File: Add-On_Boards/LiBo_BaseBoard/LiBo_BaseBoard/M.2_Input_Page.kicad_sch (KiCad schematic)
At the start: 9 parts, among them J2 2199230-3

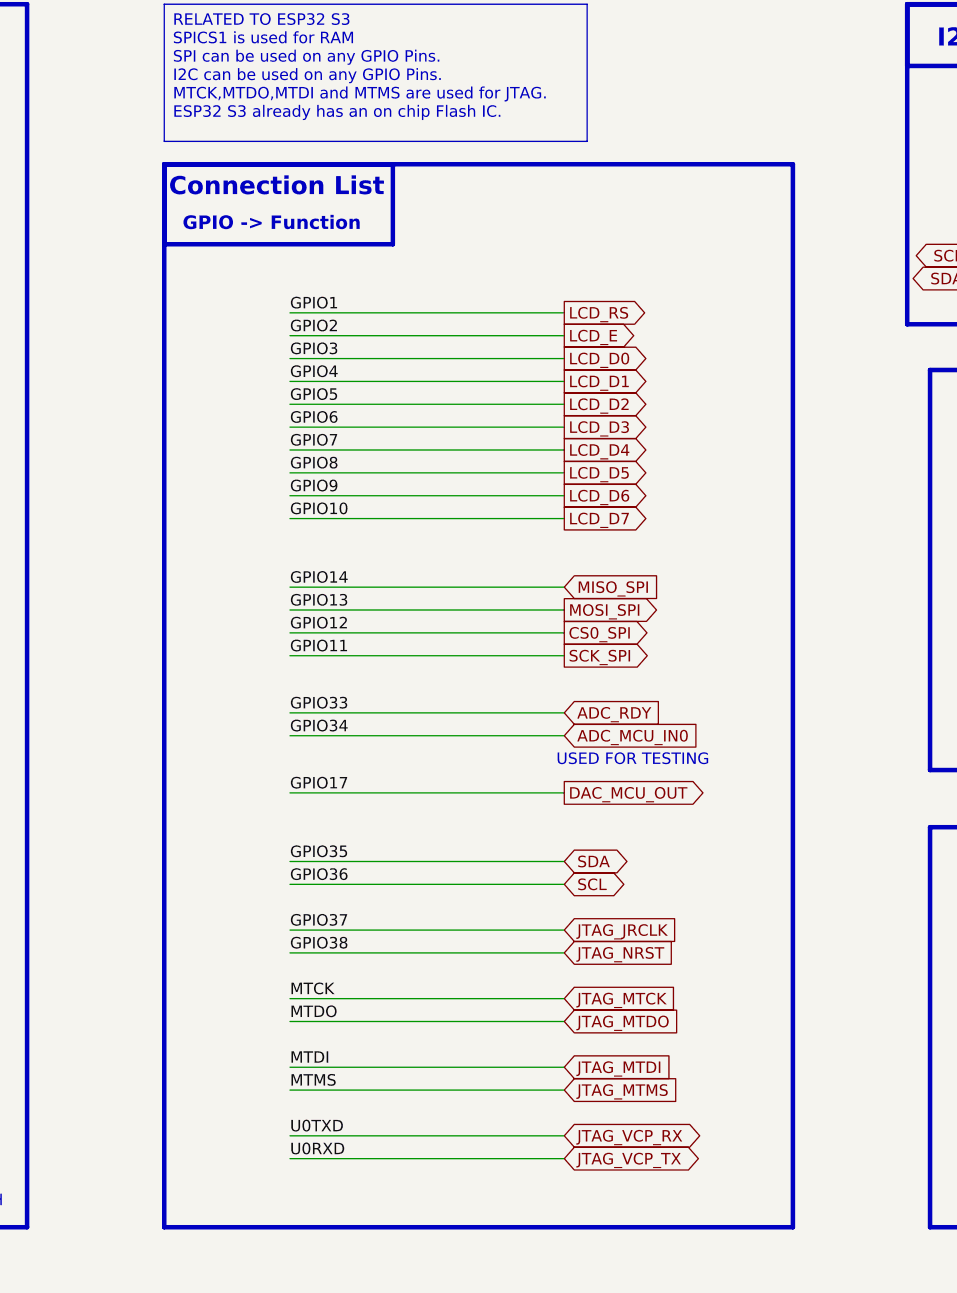
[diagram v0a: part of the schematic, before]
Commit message: first release
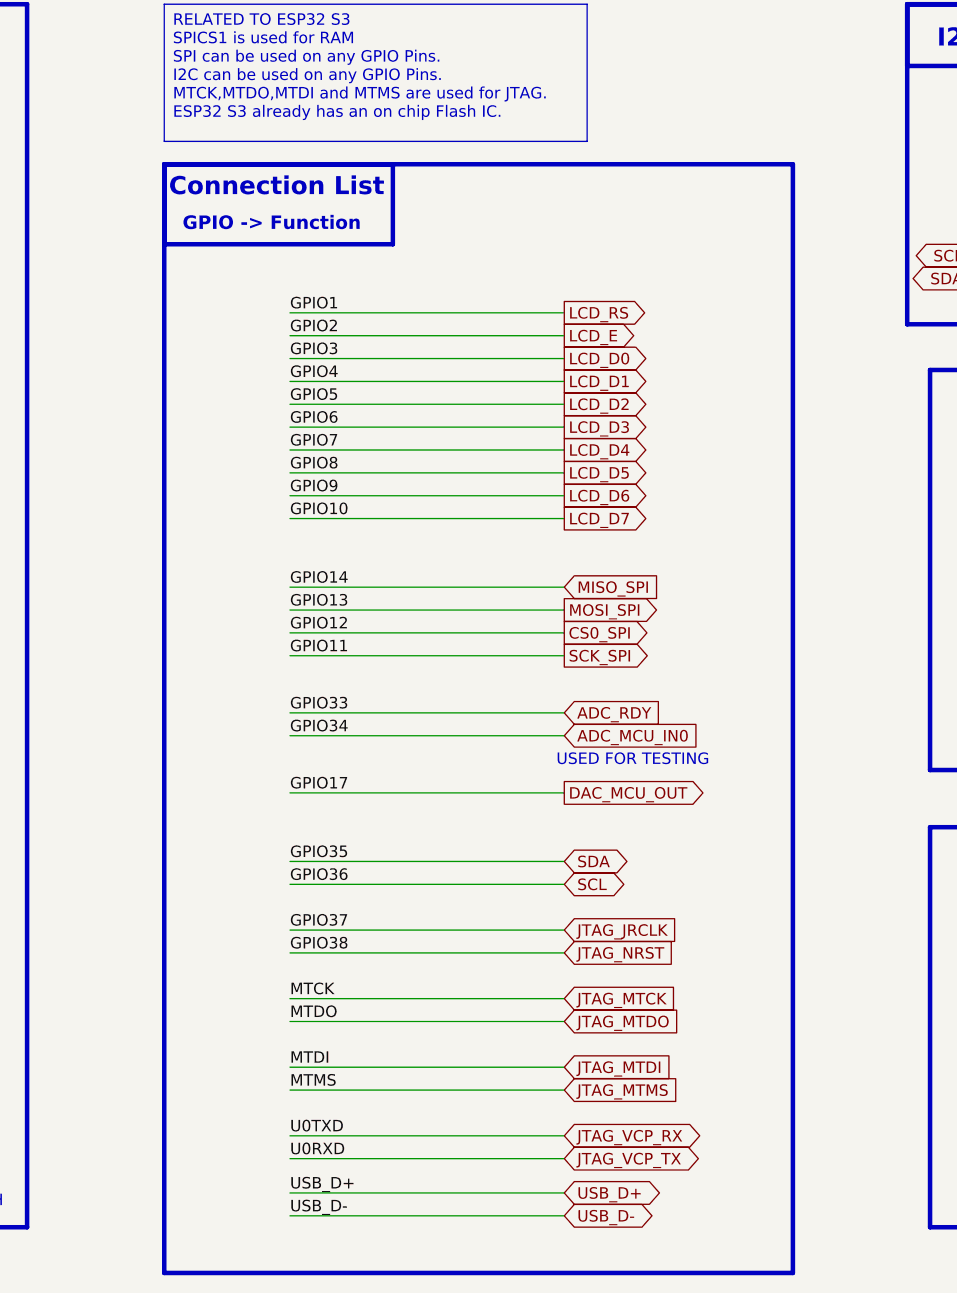
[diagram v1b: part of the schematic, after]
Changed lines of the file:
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@@
 	(rectangle
 		(start 128.27 39.37)
-		(end 198.12 157.48)
+		(end 198.12 162.56)
 		(stroke
 			(width 0.5)
@@
 	(wire
 		(pts
+			(xy 142.24 153.67) (xy 172.72 153.67)
+		)
+		(stroke
+			(width 0)
+			(type default)
+		)
+	)
+	(wire
+		(pts
 			(xy 81.28 80.01) (xy 81.28 72.39)
 		)
@@
 		(pts
 			(xy 53.34 52.07) (xy 53.34 54.61)
+		)
+		(stroke
+			(width 0)
+			(type default)
+		)
+	)
+	(wire
+		(pts
+			(xy 142.24 156.21) (xy 172.72 156.21)
 		)
 		(stroke
@@
 		)
 	)
+	(label "USB_D+"
+		(at 142.24 153.67 0)
+		(effects
+			(font
+				(size 1.27 1.27)
+			)
+			(justify left bottom)
+		)
+	)
 	(label "SDA"
 		(at 219.71 52.07 0)
@@
 	(label "GPIO7"
 		(at 142.24 71.12 0)
+		(effects
+			(font
+				(size 1.27 1.27)
+			)
+			(justify left bottom)
+		)
+	)
+	(label "USB_D-"
+		(at 142.24 156.21 0)
 		(effects
 			(font
@@
 		)
 	)
+	(global_label "USB_D+"
+		(shape bidirectional)
+		(at 172.72 153.67 0)
+		(fields_autoplaced yes)
+		(effects
+			(font
+				(size 1.27 1.27)
+			)
+			(justify left)
+		)
+		(property "Intersheetrefs" "${INTERSHEET_REFS}"
+			(at 183.3252 153.67 0)
+			(effects
+				(font
+					(size 1.27 1.27)
+				)
+				(justify left)
+				(hide yes)
+			)
+		)
+	)
 	(global_label "JTAG_VCP_RX"
 		(shape bidirectional)
@@
 			(effects
 				(font
+					(size 1.27 1.27)
+				)
+				(justify left)
+				(hide yes)
+			)
+		)
+	)
+	(global_label "USB_D-"
+		(shape bidirectional)
+		(at 172.72 156.21 0)
+		(fields_autoplaced yes)
+		(effects
+			(font
+				(size 1.27 1.27)
+			)
+			(justify left)
+		)
+		(property "Intersheetrefs" "${INTERSHEET_REFS}"
+			(at 183.3252 156.21 0)
+			(effects
+				(font
